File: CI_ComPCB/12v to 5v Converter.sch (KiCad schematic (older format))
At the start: 17 parts, among them IC401 TPS54331DR, J401 Connector_Conn_01x02_Male, J402 Connector_Conn_01x02_Male

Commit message: V1.1 Rough
Almost complete
needs silk screen annotations then will be ready to have printed
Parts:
- D401, D402: symbol SamacSys_Parts:SS34 -> CI_ComPCB-rescue:SS34-SamacSys_Parts
- IC401: symbol SamacSys_Parts:TPS54331DR -> CI_ComPCB-rescue:TPS54331DR-SamacSys_Parts
- J401, J402: symbol CI_ComPCB-cache:Connector_Conn_01x02_Male -> CI_ComPCB-rescue:Connector_Conn_01x02_Male-CI_ComPCB-cache
- L401: symbol SamacSys_Parts:RLF12560T-7R8N8R2 -> CI_ComPCB-rescue:RLF12560T-7R8N8R2-SamacSys_Parts
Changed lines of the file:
@@
 Buck_IN
 $Comp
-L CI_ComPCB-cache:Connector_Conn_01x02_Male J402
+L CI_ComPCB-rescue:Connector_Conn_01x02_Male-CI_ComPCB-cache J402
 U 1 1 6129A665
 P 8100 2650
+AR Path="/6129A665" Ref="J402"  Part="1"
+AR Path="/61A31DC2/6129A665" Ref="J402"  Part="1"
 F 0 "J402" V 8162 2694 50  0000 L CNN
 F 1 "Connector_Conn_01x02_Male" V 8253 2694 50  0000 L CNN
@@
 $EndComp
 $Comp
-L CI_ComPCB-cache:Connector_Conn_01x02_Male J401
+L CI_ComPCB-rescue:Connector_Conn_01x02_Male-CI_ComPCB-cache J401
 U 1 1 6129C94F
 P 3210 3450
+AR Path="/6129C94F" Ref="J401"  Part="1"
+AR Path="/61A31DC2/6129C94F" Ref="J401"  Part="1"
 F 0 "J401" V 3272 3494 50  0000 L CNN
 F 1 "Connector_Conn_01x02_Male" V 3363 3494 50  0000 L CNN
@@
 $EndComp
 $Comp
-L SamacSys_Parts:SS34 D402
+L CI_ComPCB-rescue:SS34-SamacSys_Parts D402
 U 1 1 612967EC
 P 8100 2850
@@
 	5600 3650 5850 3650
 $Comp
-L SamacSys_Parts:SS34 D401
+L CI_ComPCB-rescue:SS34-SamacSys_Parts D401
 U 1 1 6129D4B6
 P 5850 2900
@@
 	7400 2850 7400 3440
 $Comp
-L SamacSys_Parts:RLF12560T-7R8N8R2 L401
+L CI_ComPCB-rescue:RLF12560T-7R8N8R2-SamacSys_Parts L401
 U 1 1 612ACFD5
 P 5850 2850
@@
 Connection ~ 6650 2850
 $Comp
-L SamacSys_Parts:TPS54331DR IC401
+L CI_ComPCB-rescue:TPS54331DR-SamacSys_Parts IC401
 U 1 1 612C5C0D
 P 4400 3550

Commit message: V1.1 board
Board is ready to print
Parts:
- IC401: footprint SOIC127P600X175-8N -> SamacSys_Parts:SOIC127P600X175-8N
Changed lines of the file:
@@
 F 0 "IC401" H 5000 3815 50  0000 C CNN
 F 1 "TPS54331DR" H 5000 3724 50  0000 C CNN
-F 2 "SOIC127P600X175-8N" H 5450 3650 50  0001 L CNN
+F 2 "SamacSys_Parts:SOIC127P600X175-8N" H 5450 3650 50  0001 L CNN
 F 3 "http://www.ti.com/lit/gpn/tps54331" H 5450 3550 50  0001 L CNN
 F 4 "Texas Instruments TPS54331DR, Step Down DC-DC Converter, 3A, Adjustable, 0.8  25 V, 8-Pin SOIC" H 5450 3450 50  0001 L CNN "Description"

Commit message: V1.1 Changed Diode for reprint
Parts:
- D401, D402: footprint SamacSys_Parts:DIOM8059X256N -> digikey-footprints:DO-214AC
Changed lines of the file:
@@
 F 0 "D402" H 8500 2583 50  0000 C CNN
 F 1 "SS34" H 8500 2674 50  0000 C CNN
-F 2 "SamacSys_Parts:DIOM8059X256N" H 8600 3000 50  0001 L CNN
+F 2 "digikey-footprints:DO-214AC" H 8600 3000 50  0001 L CNN
 F 3 "https://componentsearchengine.com/Datasheets/2/SS34.pdf" H 8600 2900 50  0001 L CNN
 F 4 "ON Semi SS34 SMT Schottky Diode, 40V 3A, 2-Pin DO-214AB" H 8600 2800 50  0001 L CNN "Description"
@@
 F 0 "D401" H 6250 2633 50  0000 C CNN
 F 1 "SS34" H 6250 2724 50  0000 C CNN
-F 2 "SamacSys_Parts:DIOM8059X256N" H 6350 3050 50  0001 L CNN
+F 2 "digikey-footprints:DO-214AC" H 6350 3050 50  0001 L CNN
 F 3 "https://componentsearchengine.com/Datasheets/2/SS34.pdf" H 6350 2950 50  0001 L CNN
 F 4 "ON Semi SS34 SMT Schottky Diode, 40V 3A, 2-Pin DO-214AB" H 6350 2850 50  0001 L CNN "Description"

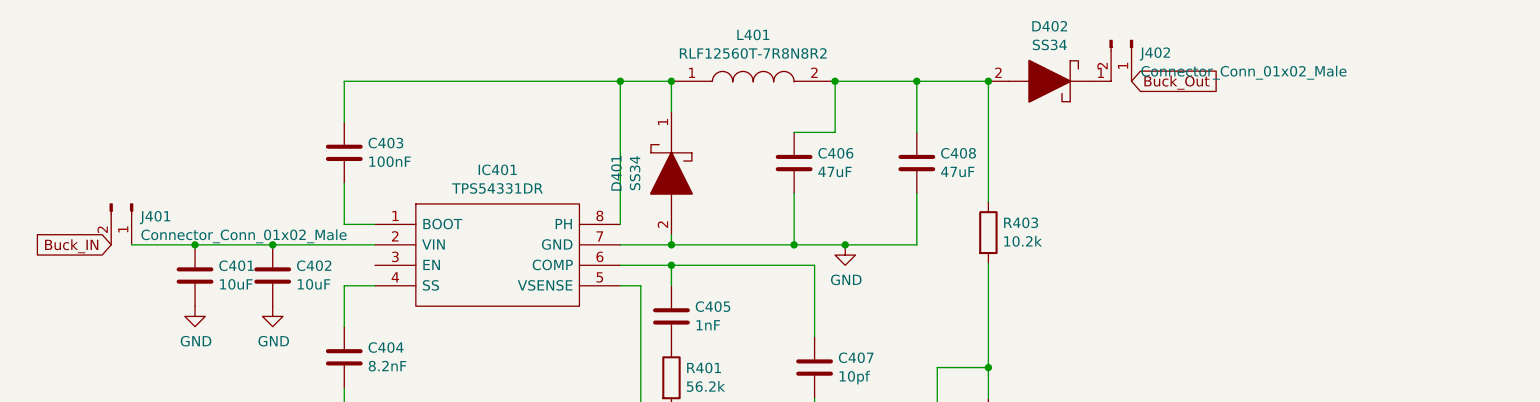
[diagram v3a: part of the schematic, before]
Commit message: switch
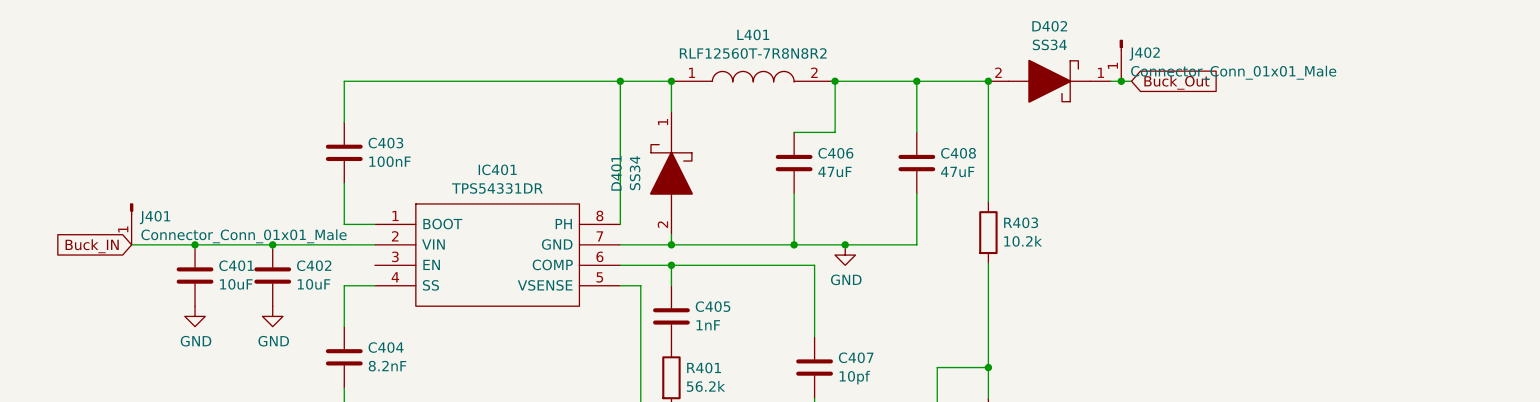
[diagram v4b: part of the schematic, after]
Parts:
- removed J401, J402: Connector_Conn_01x02_Male, Connector_PinHeader_2.54mm:PinHeader_1x02_P2.54mm_Vertical, symbol CI_ComPCB-rescue:Connector_Conn_01x02_Male-CI_ComPCB-cache
- added J401, J402: Connector_Conn_01x01_Male, Connector_PinHeader_2.54mm:PinHeader_1x01_P2.54mm_Vertical, symbol CI_ComPCB-cache:Connector_Conn_01x01_Male
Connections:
- net Buck_IN: now also C401.1, C402.1, IC401.2 (VIN), J401.1 (Pin_1)
- net Buck_Out: now also D402.1, J402.1 (Pin_1)
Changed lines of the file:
@@
 	7050 3100 7050 2850
 Connection ~ 6450 3650
-Wire Wire Line
-	6450 3650 6700 3650
-$Comp
-L power:GND #PWR?
-U 1 1 61A8D150
-P 6700 3650
-AR Path="/61A8D150" Ref="#PWR?"  Part="1"
-AR Path="/61A31DC2/61A8D150" Ref="#PWR0405"  Part="1"
-F 0 "#PWR0405" H 6700 3400 50  0001 C CNN
-F 1 "GND" H 6705 3477 50  0000 C CNN
-F 2 "" H 6700 3650 50  0001 C CNN
-F 3 "" H 6700 3650 50  0001 C CNN
-	1    6700 3650
-	1    0    0    -1
-$EndComp
-Connection ~ 6700 3650
-Wire Wire Line
-	6700 3650 7050 3650
 $Comp
 L Device:C C?
@@
 	1    0    0    -1
 $EndComp
-Wire Wire Line
-	5850 4450 5850 4700
-Wire Wire Line
-	5850 4700 6200 4700
-Wire Wire Line
-	6550 4700 6550 4400
-$Comp
-L power:GND #PWR?
-U 1 1 61A8D172
-P 6200 4700
-AR Path="/61A8D172" Ref="#PWR?"  Part="1"
-AR Path="/61A31DC2/61A8D172" Ref="#PWR0404"  Part="1"
-F 0 "#PWR0404" H 6200 4450 50  0001 C CNN
-F 1 "GND" H 6205 4527 50  0000 C CNN
-F 2 "" H 6200 4700 50  0001 C CNN
-F 3 "" H 6200 4700 50  0001 C CNN
-	1    6200 4700
-	1    0    0    -1
-$EndComp
-Connection ~ 6200 4700
-Wire Wire Line
-	6200 4700 6550 4700
 $Comp
 L Device:R R?
@@
 	1    0    0    -1
 $EndComp
-$Comp
-L Device:R R?
-U 1 1 61A8D180
-P 7400 4550
-AR Path="/61A8D180" Ref="R?"  Part="1"
-AR Path="/61A31DC2/61A8D180" Ref="R404"  Part="1"
-F 0 "R404" H 7470 4596 50  0000 L CNN
-F 1 "1.78k" H 7470 4505 50  0000 L CNN
-F 2 "Resistor_SMD:R_0805_2012Metric" V 7330 4550 50  0001 C CNN
-F 3 "~" H 7400 4550 50  0001 C CNN
-	1    7400 4550
-	1    0    0    -1
-$EndComp
 Wire Wire Line
 	5600 3850 5700 3850
-Wire Wire Line
-	5700 4950 7150 4950
-Wire Wire Line
-	7150 4950 7150 4250
-Wire Wire Line
-	7150 4250 7400 4250
-Wire Wire Line
-	7400 4250 7400 4400
-Wire Wire Line
-	7400 3740 7400 4250
-Connection ~ 7400 4250
-$Comp
-L power:GND #PWR?
-U 1 1 61A8D18E
-P 7400 4900
-AR Path="/61A8D18E" Ref="#PWR?"  Part="1"
-AR Path="/61A31DC2/61A8D18E" Ref="#PWR0406"  Part="1"
-F 0 "#PWR0406" H 7400 4650 50  0001 C CNN
-F 1 "GND" H 7405 4727 50  0000 C CNN
-F 2 "" H 7400 4900 50  0001 C CNN
-F 3 "" H 7400 4900 50  0001 C CNN
-	1    7400 4900
-	1    0    0    -1
-$EndComp
-Wire Wire Line
-	7400 4700 7400 4900
 $Comp
 L Device:C C?
@@
 	1    0    0    -1
 $EndComp
-$Comp
-L power:GND #PWR?
-U 1 1 61A8D1A1
-P 4250 4550
-AR Path="/61A8D1A1" Ref="#PWR?"  Part="1"
-AR Path="/61A31DC2/61A8D1A1" Ref="#PWR0403"  Part="1"
-F 0 "#PWR0403" H 4250 4300 50  0001 C CNN
-F 1 "GND" H 4255 4377 50  0000 C CNN
-F 2 "" H 4250 4550 50  0001 C CNN
-F 3 "" H 4250 4550 50  0001 C CNN
-	1    4250 4550
-	1    0    0    -1
-$EndComp
-Wire Wire Line
-	4250 4350 4250 4550
 Wire Wire Line
 	4250 4050 4250 3850
-$Comp
-L power:GND #PWR?
-U 1 1 61A8D1AA
-P 3900 3950
-AR Path="/61A8D1AA" Ref="#PWR?"  Part="1"
-AR Path="/61A31DC2/61A8D1AA" Ref="#PWR0402"  Part="1"
-F 0 "#PWR0402" H 3900 3700 50  0001 C CNN
-F 1 "GND" H 3905 3777 50  0000 C CNN
-F 2 "" H 3900 3950 50  0001 C CNN
-F 3 "" H 3900 3950 50  0001 C CNN
-	1    3900 3950
-	1    0    0    -1
-$EndComp
 Connection ~ 3900 3650
 Wire Wire Line
@@
 	1    0    0    -1
 $EndComp
-$Comp
-L power:GND #PWR?
-U 1 1 61A8D1BC
-P 3520 3950
-AR Path="/61A8D1BC" Ref="#PWR?"  Part="1"
-AR Path="/61A31DC2/61A8D1BC" Ref="#PWR0401"  Part="1"
-F 0 "#PWR0401" H 3520 3700 50  0001 C CNN
-F 1 "GND" H 3525 3777 50  0000 C CNN
-F 2 "" H 3520 3950 50  0001 C CNN
-F 3 "" H 3520 3950 50  0001 C CNN
-	1    3520 3950
-	1    0    0    -1
-$EndComp
 Wire Wire Line
 	5600 2850 5850 2850
@@
 Wire Wire Line
 	3520 3650 3900 3650
-Text GLabel 3110 3650 0    50   Input ~ 0
+Text GLabel 3210 3650 0    50   Input ~ 0
 Buck_IN
-$Comp
-L CI_ComPCB-rescue:Connector_Conn_01x02_Male-CI_ComPCB-cache J402
-U 1 1 6129A665
-P 8100 2650
-AR Path="/6129A665" Ref="J402"  Part="1"
-AR Path="/61A31DC2/6129A665" Ref="J402"  Part="1"
-F 0 "J402" V 8162 2694 50  0000 L CNN
-F 1 "Connector_Conn_01x02_Male" V 8253 2694 50  0000 L CNN
-F 2 "Connector_PinHeader_2.54mm:PinHeader_1x02_P2.54mm_Vertical" H 8100 2650 50  0001 C CNN
-F 3 "" H 8100 2650 50  0001 C CNN
-	1    8100 2650
-	0    1    1    0
-$EndComp
-$Comp
-L CI_ComPCB-rescue:Connector_Conn_01x02_Male-CI_ComPCB-cache J401
-U 1 1 6129C94F
-P 3210 3450
-AR Path="/6129C94F" Ref="J401"  Part="1"
-AR Path="/61A31DC2/6129C94F" Ref="J401"  Part="1"
-F 0 "J401" V 3272 3494 50  0000 L CNN
-F 1 "Connector_Conn_01x02_Male" V 3363 3494 50  0000 L CNN
-F 2 "Connector_PinHeader_2.54mm:PinHeader_1x02_P2.54mm_Vertical" H 3210 3450 50  0001 C CNN
-F 3 "" H 3210 3450 50  0001 C CNN
-	1    3210 3450
-	0    1    1    0
-$EndComp
 $Comp
 L CI_ComPCB-rescue:SS34-SamacSys_Parts D402
@@
 Wire Wire Line
 	4250 3550 4400 3550
+Wire Wire Line
+	6450 3650 6700 3650
+Connection ~ 6700 3650
+$Comp
+L power:GND #PWR?
+U 1 1 61A8D150
+P 6700 3650
+AR Path="/61A8D150" Ref="#PWR?"  Part="1"
+AR Path="/61A31DC2/61A8D150" Ref="#PWR0405"  Part="1"
+F 0 "#PWR0405" H 6700 3400 50  0001 C CNN
+F 1 "GND" H 6705 3477 50  0000 C CNN
+F 2 "" H 6700 3650 50  0001 C CNN
+F 3 "" H 6700 3650 50  0001 C CNN
+	1    6700 3650
+	1    0    0    -1
+$EndComp
+Wire Wire Line
+	6700 3650 7050 3650
+Connection ~ 6200 4700
+Wire Wire Line
+	6200 4700 6550 4700
+Wire Wire Line
+	5850 4700 6200 4700
+$Comp
+L power:GND #PWR?
+U 1 1 61A8D172
+P 6200 4700
+AR Path="/61A8D172" Ref="#PWR?"  Part="1"
+AR Path="/61A31DC2/61A8D172" Ref="#PWR0404"  Part="1"
+F 0 "#PWR0404" H 6200 4450 50  0001 C CNN
+F 1 "GND" H 6205 4527 50  0000 C CNN
+F 2 "" H 6200 4700 50  0001 C CNN
+F 3 "" H 6200 4700 50  0001 C CNN
+	1    6200 4700
+	1    0    0    -1
+$EndComp
+Wire Wire Line
+	5700 4950 7150 4950
+Wire Wire Line
+	7400 4700 7400 4900
+$Comp
+L power:GND #PWR?
+U 1 1 61A8D18E
+P 7400 4900
+AR Path="/61A8D18E" Ref="#PWR?"  Part="1"
+AR Path="/61A31DC2/61A8D18E" Ref="#PWR0406"  Part="1"
+F 0 "#PWR0406" H 7400 4650 50  0001 C CNN
+F 1 "GND" H 7405 4727 50  0000 C CNN
+F 2 "" H 7400 4900 50  0001 C CNN
+F 3 "" H 7400 4900 50  0001 C CNN
+	1    7400 4900
+	1    0    0    -1
+$EndComp
+Wire Wire Line
+	7400 3740 7400 4250
+Wire Wire Line
+	7400 4250 7400 4400
+Connection ~ 7400 4250
+Wire Wire Line
+	7150 4250 7400 4250
+Wire Wire Line
+	7150 4950 7150 4250
+Wire Wire Line
+	6550 4700 6550 4400
+$Comp
+L Device:R R?
+U 1 1 61A8D180
+P 7400 4550
+AR Path="/61A8D180" Ref="R?"  Part="1"
+AR Path="/61A31DC2/61A8D180" Ref="R404"  Part="1"
+F 0 "R404" H 7470 4596 50  0000 L CNN
+F 1 "1.78k" H 7470 4505 50  0000 L CNN
+F 2 "Resistor_SMD:R_0805_2012Metric" V 7330 4550 50  0001 C CNN
+F 3 "~" H 7400 4550 50  0001 C CNN
+	1    7400 4550
+	1    0    0    -1
+$EndComp
+Wire Wire Line
+	5850 4450 5850 4700
+$Comp
+L power:GND #PWR?
+U 1 1 61A8D1A1
+P 4250 4550
+AR Path="/61A8D1A1" Ref="#PWR?"  Part="1"
+AR Path="/61A31DC2/61A8D1A1" Ref="#PWR0403"  Part="1"
+F 0 "#PWR0403" H 4250 4300 50  0001 C CNN
+F 1 "GND" H 4255 4377 50  0000 C CNN
+F 2 "" H 4250 4550 50  0001 C CNN
+F 3 "" H 4250 4550 50  0001 C CNN
+	1    4250 4550
+	1    0    0    -1
+$EndComp
+Wire Wire Line
+	4250 4350 4250 4550
+$Comp
+L power:GND #PWR?
+U 1 1 61A8D1AA
+P 3900 3950
+AR Path="/61A8D1AA" Ref="#PWR?"  Part="1"
+AR Path="/61A31DC2/61A8D1AA" Ref="#PWR0402"  Part="1"
+F 0 "#PWR0402" H 3900 3700 50  0001 C CNN
+F 1 "GND" H 3905 3777 50  0000 C CNN
+F 2 "" H 3900 3950 50  0001 C CNN
+F 3 "" H 3900 3950 50  0001 C CNN
+	1    3900 3950
+	1    0    0    -1
+$EndComp
+$Comp
+L power:GND #PWR?
+U 1 1 61A8D1BC
+P 3520 3950
+AR Path="/61A8D1BC" Ref="#PWR?"  Part="1"
+AR Path="/61A31DC2/61A8D1BC" Ref="#PWR0401"  Part="1"
+F 0 "#PWR0401" H 3520 3700 50  0001 C CNN
+F 1 "GND" H 3525 3777 50  0000 C CNN
+F 2 "" H 3520 3950 50  0001 C CNN
+F 3 "" H 3520 3950 50  0001 C CNN
+	1    3520 3950
+	1    0    0    -1
+$EndComp
+$Comp
+L CI_ComPCB-cache:Connector_Conn_01x01_Male J402
+U 1 1 614D6EFD
+P 8050 2650
+F 0 "J402" V 8112 2694 50  0000 L CNN
+F 1 "Connector_Conn_01x01_Male" V 8203 2694 50  0000 L CNN
+F 2 "Connector_PinHeader_2.54mm:PinHeader_1x01_P2.54mm_Vertical" H 8050 2650 50  0001 C CNN
+F 3 "" H 8050 2650 50  0001 C CNN
+	1    8050 2650
+	0    1    1    0
+$EndComp
+Wire Wire Line
+	8100 2850 8050 2850
+Wire Wire Line
+	8000 2850 8050 2850
+Connection ~ 8050 2850
+$Comp
+L CI_ComPCB-cache:Connector_Conn_01x01_Male J401
+U 1 1 614D9F4C
+P 3210 3450
+F 0 "J401" V 3272 3494 50  0000 L CNN
+F 1 "Connector_Conn_01x01_Male" V 3363 3494 50  0000 L CNN
+F 2 "Connector_PinHeader_2.54mm:PinHeader_1x01_P2.54mm_Vertical" H 3210 3450 50  0001 C CNN
+F 3 "" H 3210 3450 50  0001 C CNN
+	1    3210 3450
+	0    1    1    0
+$EndComp
 $EndSCHEMATC

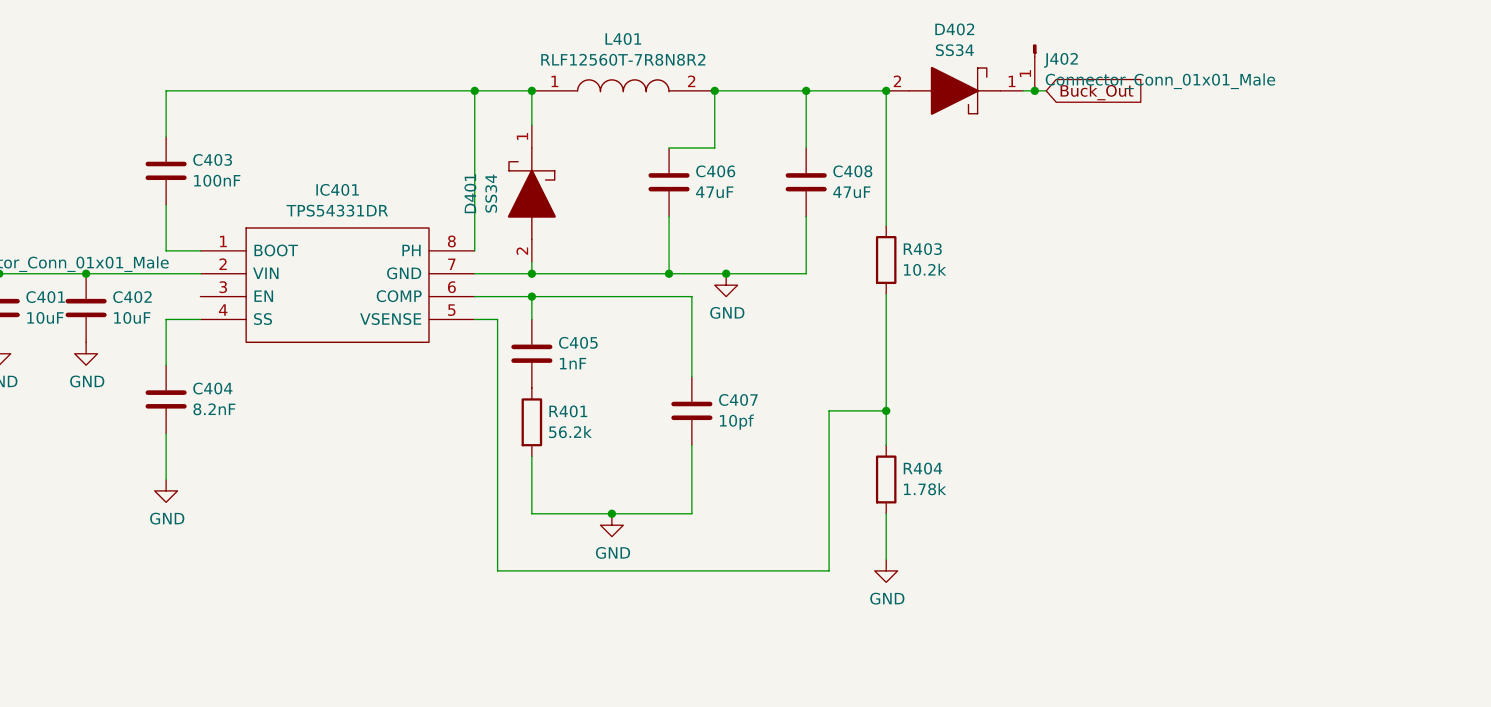
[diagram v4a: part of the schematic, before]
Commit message: Ready to Build
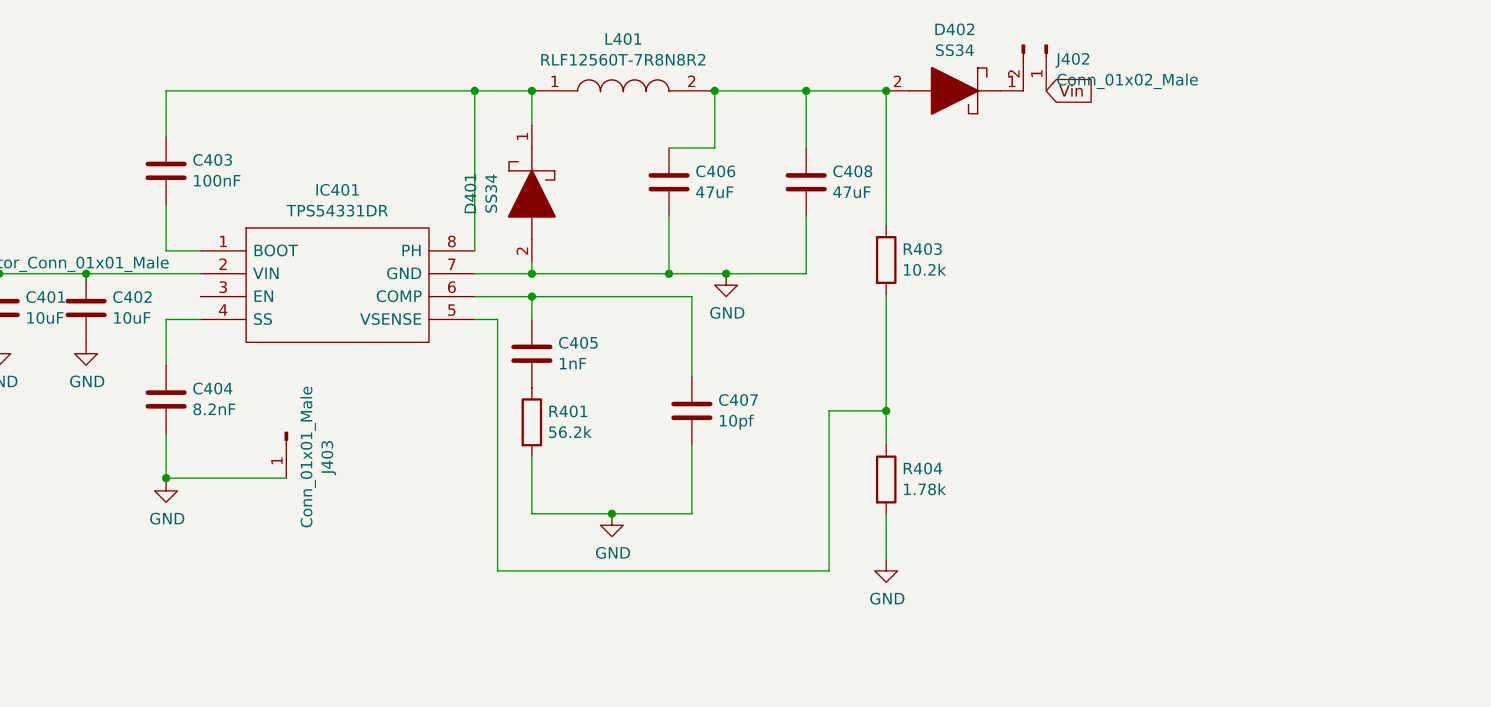
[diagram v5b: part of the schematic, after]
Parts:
- removed J402: Connector_Conn_01x01_Male, Connector_PinHeader_2.54mm:PinHeader_1x01_P2.54mm_Vertical, symbol CI_ComPCB-cache:Connector_Conn_01x01_Male
- added J402: Conn_01x02_Male, Connector_PinHeader_2.54mm:PinHeader_1x02_P2.54mm_Vertical, symbol Connector:Conn_01x02_Male
- added J403: Conn_01x01_Male, Connector_PinHeader_2.54mm:PinHeader_1x01_P2.54mm_Vertical, symbol Connector:Conn_01x01_Male
- C404: footprint Capacitor_SMD:C_0805_2012Metric -> Capacitor_SMD:C_0603_1608Metric
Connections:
- net GND: now also J403.1 (Pin_1)
- net Buck_Out: no longer names the net of D402.1
- net Buck_Out: now also J402.2 (Pin_2)
- new net Vin: J402.1 (Pin_1)
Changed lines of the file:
@@
 $Descr A4 11693 8268
 encoding utf-8
-Sheet 4 5
+Sheet 4 6
 Title ""
 Date ""
@@
 F 0 "C404" H 4365 4246 50  0000 L CNN
 F 1 "8.2nF" H 4365 4155 50  0000 L CNN
-F 2 "Capacitor_SMD:C_0805_2012Metric" H 4288 4050 50  0001 C CNN
+F 2 "Capacitor_SMD:C_0603_1608Metric" H 4288 4050 50  0001 C CNN
 F 3 "https://datasheet.lcsc.com/lcsc/1811071710_Sunlord-SDCL1608C8N2JTDF_C1032.pdf" H 4250 4200 50  0001 C CNN
 F 4 "C1032" H 4250 4200 50  0001 C CNN "JLCPCB"
@@
 12v to 5v converter
 Text GLabel 8100 2850 2    50   Input ~ 0
-Buck_Out
+Vin
 Text Notes 7060 7090 0    50   ~ 0
 https://webench.ti.com/power-designer/switching-regulator/customize/8?noparams=0
@@
 	1    0    0    -1
 $EndComp
-Wire Wire Line
-	4250 4350 4250 4550
 $Comp
 L power:GND #PWR?
@@
 $EndComp
 $Comp
-L CI_ComPCB-cache:Connector_Conn_01x01_Male J402
-U 1 1 614D6EFD
-P 8050 2650
-F 0 "J402" V 8112 2694 50  0000 L CNN
-F 1 "Connector_Conn_01x01_Male" V 8203 2694 50  0000 L CNN
-F 2 "Connector_PinHeader_2.54mm:PinHeader_1x01_P2.54mm_Vertical" H 8050 2650 50  0001 C CNN
-F 3 "" H 8050 2650 50  0001 C CNN
-	1    8050 2650
-	0    1    1    0
-$EndComp
-Wire Wire Line
-	8100 2850 8050 2850
-Wire Wire Line
-	8000 2850 8050 2850
-Connection ~ 8050 2850
-$Comp
 L CI_ComPCB-cache:Connector_Conn_01x01_Male J401
 U 1 1 614D9F4C
@@
 	0    1    1    0
 $EndComp
+$Comp
+L Connector:Conn_01x02_Male J402
+U 1 1 61839510
+P 8100 2650
+F 0 "J402" V 8162 2694 50  0000 L CNN
+F 1 "Conn_01x02_Male" V 8253 2694 50  0000 L CNN
+F 2 "Connector_PinHeader_2.54mm:PinHeader_1x02_P2.54mm_Vertical" H 8100 2650 50  0001 C CNN
+F 3 "~" H 8100 2650 50  0001 C CNN
+	1    8100 2650
+	0    1    1    0
+$EndComp
+$Comp
+L Connector:Conn_01x01_Male J403
+U 1 1 6184D048
+P 4776 4344
+F 0 "J403" H 4884 4525 50  0000 C CNN
+F 1 "Conn_01x01_Male" H 4884 4434 50  0000 C CNN
+F 2 "Connector_PinHeader_2.54mm:PinHeader_1x01_P2.54mm_Vertical" H 4776 4344 50  0001 C CNN
+F 3 "~" H 4776 4344 50  0001 C CNN
+	1    4776 4344
+	0    1    1    0
+$EndComp
+Wire Wire Line
+	4776 4544 4250 4544
+Wire Wire Line
+	4250 4350 4250 4544
+Connection ~ 4250 4544
+Wire Wire Line
+	4250 4544 4250 4550
 $EndSCHEMATC
